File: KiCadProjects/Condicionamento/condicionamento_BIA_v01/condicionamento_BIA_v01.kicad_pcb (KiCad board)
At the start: 2 copper layers, 90 x 100 mm, 27 parts, among them J1 Vref, J2 tensoes, J3 sinais analogicos, J4 comunicacao / sinais digitais, J5 sinais_condicionados, J6 Vmaster, J7 Eletrodos, U1 AD828AN, U2 BluePill_STM32F103C, U3 BluePill_STM32F103C_master

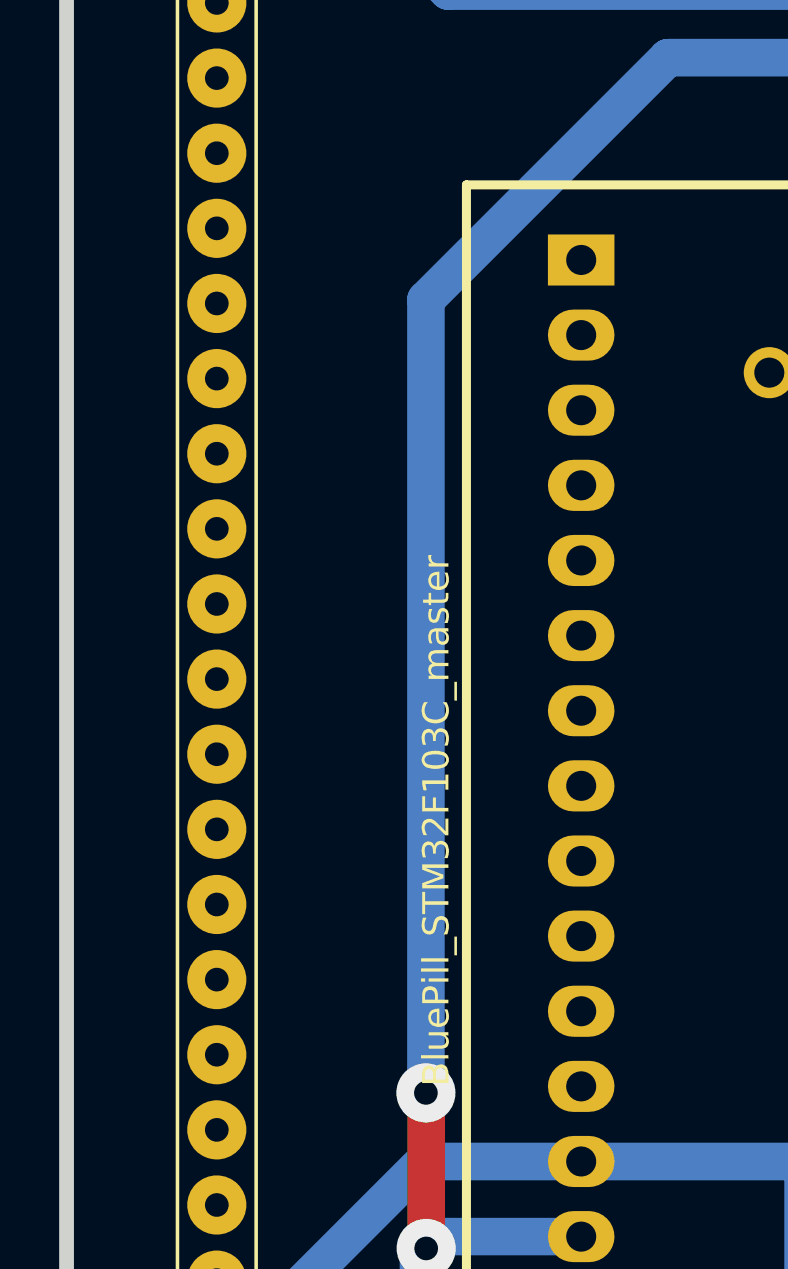
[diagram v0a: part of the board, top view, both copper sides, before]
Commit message: PCB
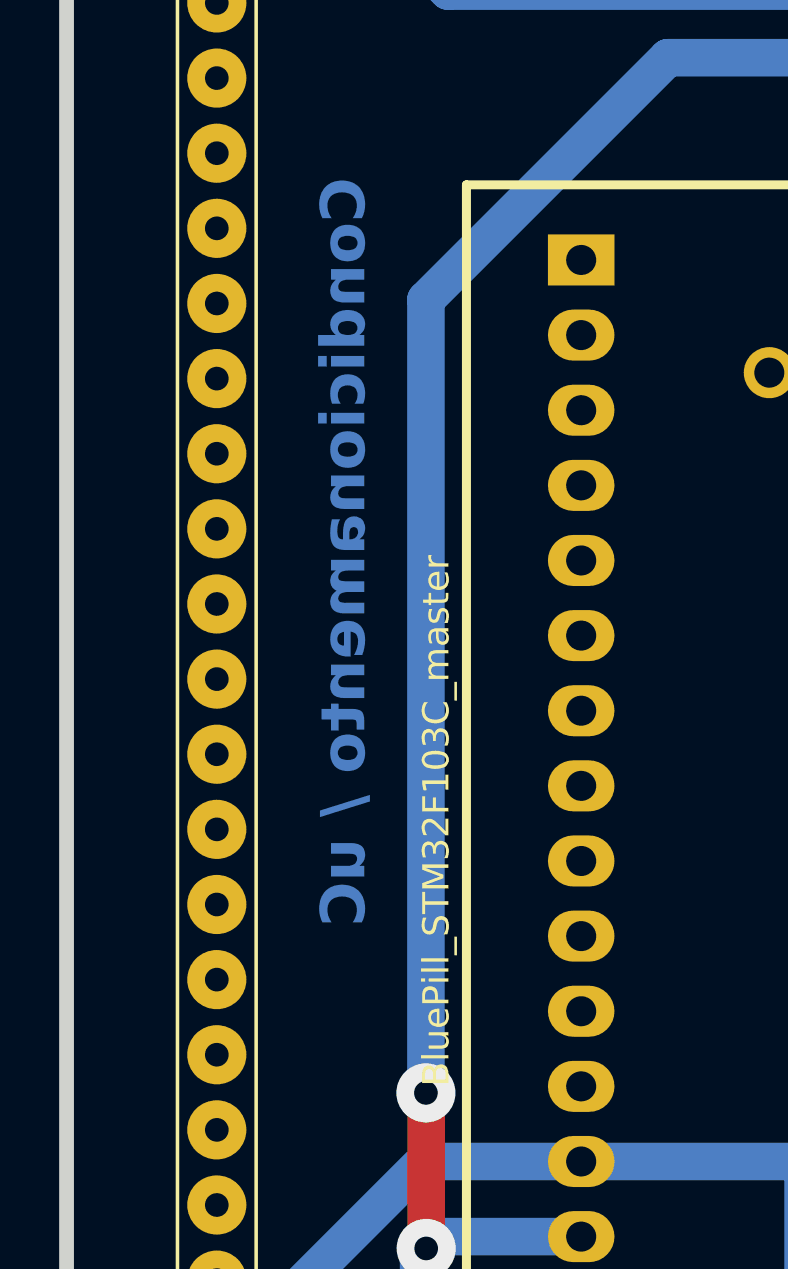
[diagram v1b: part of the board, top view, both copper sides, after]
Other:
- board text added: "Condicionamento / uC"
- board text added: "Condicionamento / uC V01 - 2023"
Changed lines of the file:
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@@
       (drillshape 0)
       (scaleselection 1)
-      (outputdirectory "gerber/drill/")
+      (outputdirectory "../gerber/drill/")
     )
   )
@@
   (gr_line (start 88.5 48.5) (end 88.5 148.4998)
     (stroke (width 0.5) (type default)) (layer "Edge.Cuts"))
+  (gr_text "Condicionamento / uC" (at 98.75 92.5 90) (layer "B.Cu")
+    (effects (font (size 1.5 1.5) (thickness 0.3) bold) (justify left bottom mirror))
+  )
+  (gr_text "Condicionamento / uC\nV01 - 2023" (at 150 119.25) (layer "B.SilkS")
+    (effects (font (size 1.5 1.5) (thickness 0.3) bold) (justify bottom))
+  )
   (gr_text "+3.3V | +5.0V" (at 102.75 79.75 90) (layer "F.SilkS")
     (effects (font (size 1.016 1.016) (thickness 0.254) bold) (justify bottom))
